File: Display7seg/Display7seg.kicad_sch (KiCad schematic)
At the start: 6 parts

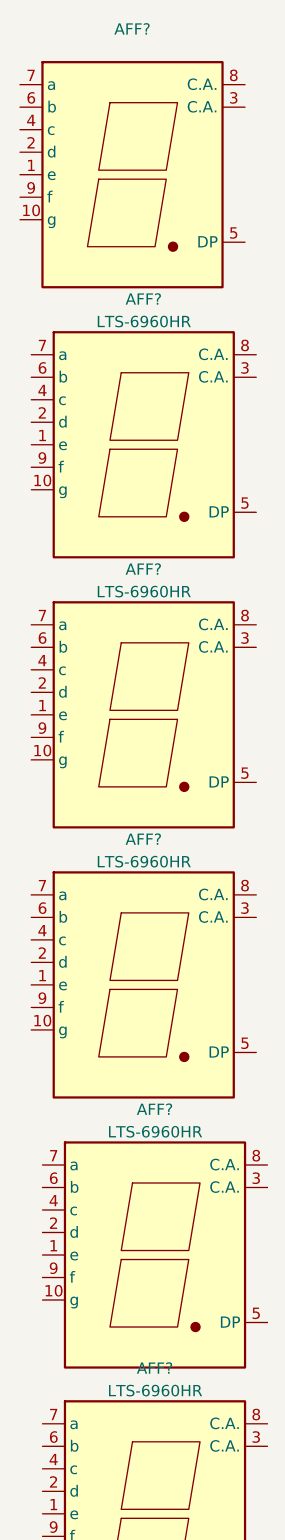
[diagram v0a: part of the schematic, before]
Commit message: Display
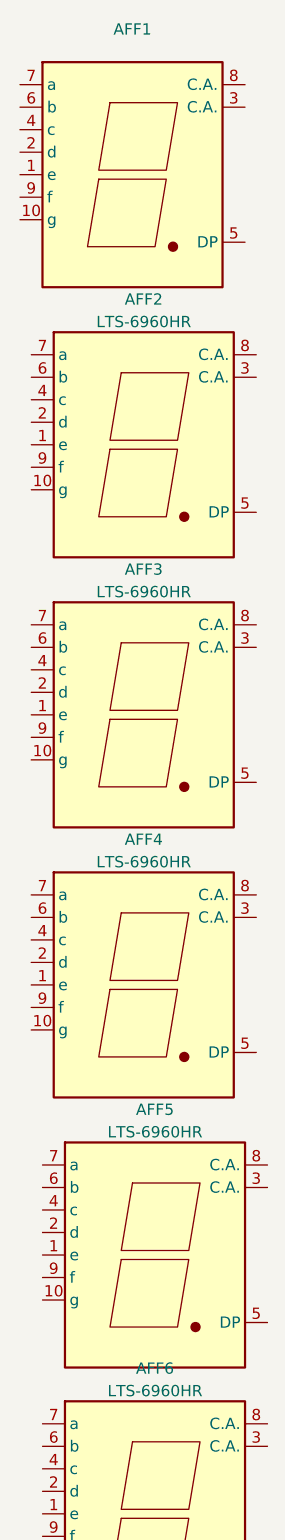
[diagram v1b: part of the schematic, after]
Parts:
- gave numbers to parts that had none: 6
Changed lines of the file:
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@@
   (symbol (lib_id "Display_Character:LTS-6960HR") (at 120.65 152.4 0) (unit 1)
     (in_bom yes) (on_board yes) (fields_autoplaced)
-    (property "Reference" "AFF?" (id 0) (at 120.65 136.0002 0))
+    (property "Reference" "AFF5" (id 0) (at 120.65 136.0002 0))
     (property "Value" "LTS-6960HR" (id 1) (at 120.65 138.5371 0))
     (property "Footprint" "Display_7Segment:7SegmentLED_LTS6760_LTS6780" (id 2) (at 120.65 167.64 0)
@@
   (symbol (lib_id "Display_Character:LTS-6960HR") (at 119.38 60.96 0) (unit 1)
     (in_bom yes) (on_board yes) (fields_autoplaced)
-    (property "Reference" "AFF?" (id 0) (at 119.38 44.5602 0))
+    (property "Reference" "AFF2" (id 0) (at 119.38 44.5602 0))
     (property "Value" "LTS-6960HR" (id 1) (at 119.38 47.0971 0))
     (property "Footprint" "Display_7Segment:7SegmentLED_LTS6760_LTS6780" (id 2) (at 119.38 76.2 0)
@@
   (symbol (lib_id "Display_Character:LTS-6960HR") (at 120.65 181.61 0) (unit 1)
     (in_bom yes) (on_board yes) (fields_autoplaced)
-    (property "Reference" "AFF?" (id 0) (at 120.65 165.2102 0))
+    (property "Reference" "AFF6" (id 0) (at 120.65 165.2102 0))
     (property "Value" "LTS-6960HR" (id 1) (at 120.65 167.7471 0))
     (property "Footprint" "Display_7Segment:7SegmentLED_LTS6760_LTS6780" (id 2) (at 120.65 196.85 0)
@@
   (symbol (lib_id "Display_Character:LTS-6960HR") (at 119.38 91.44 0) (unit 1)
     (in_bom yes) (on_board yes) (fields_autoplaced)
-    (property "Reference" "AFF?" (id 0) (at 119.38 75.0402 0))
+    (property "Reference" "AFF3" (id 0) (at 119.38 75.0402 0))
     (property "Value" "LTS-6960HR" (id 1) (at 119.38 77.5771 0))
     (property "Footprint" "Display_7Segment:7SegmentLED_LTS6760_LTS6780" (id 2) (at 119.38 106.68 0)
@@
   (symbol (lib_id "Display_Character:LTS-6960HR") (at 118.11 30.48 0) (unit 1)
     (in_bom yes) (on_board yes) (fields_autoplaced)
-    (property "Reference" "AFF?" (id 0) (at 118.11 14.0802 0))
+    (property "Reference" "AFF1" (id 0) (at 118.11 14.0802 0))
     (property "Value" "" (id 1) (at 118.11 16.6171 0))
     (property "Footprint" "" (id 2) (at 118.11 45.72 0)
@@
   (symbol (lib_id "Display_Character:LTS-6960HR") (at 119.38 121.92 0) (unit 1)
     (in_bom yes) (on_board yes) (fields_autoplaced)
-    (property "Reference" "AFF?" (id 0) (at 119.38 105.5202 0))
+    (property "Reference" "AFF4" (id 0) (at 119.38 105.5202 0))
     (property "Value" "LTS-6960HR" (id 1) (at 119.38 108.0571 0))
     (property "Footprint" "Display_7Segment:7SegmentLED_LTS6760_LTS6780" (id 2) (at 119.38 137.16 0)
@@
   )
   (symbol_instances
-    (path "/037e3cea-2b4e-4a8e-b505-8a054542ddbd"
-      (reference "AFF?") (unit 1) (value "LTS-6960HR") (footprint "Display_7Segment:7SegmentLED_LTS6760_LTS6780")
+    (path "/e82a6e2d-1a74-4e83-87b6-27ce032478fa"
+      (reference "AFF1") (unit 1) (value "LTS-6960HR") (footprint "Display_7Segment:7SegmentLED_LTS6760_LTS6780")
     )
     (path "/231a3042-ec36-4c9a-bd14-ea32ea232394"
-      (reference "AFF?") (unit 1) (value "LTS-6960HR") (footprint "Display_7Segment:7SegmentLED_LTS6760_LTS6780")
+      (reference "AFF2") (unit 1) (value "LTS-6960HR") (footprint "Display_7Segment:7SegmentLED_LTS6760_LTS6780")
+    )
+    (path "/9cad7174-bb88-4cff-8061-48eaf01fef6d"
+      (reference "AFF3") (unit 1) (value "LTS-6960HR") (footprint "Display_7Segment:7SegmentLED_LTS6760_LTS6780")
+    )
+    (path "/f1ee0cd5-9267-462c-9d04-1dd00febaf6c"
+      (reference "AFF4") (unit 1) (value "LTS-6960HR") (footprint "Display_7Segment:7SegmentLED_LTS6760_LTS6780")
+    )
+    (path "/037e3cea-2b4e-4a8e-b505-8a054542ddbd"
+      (reference "AFF5") (unit 1) (value "LTS-6960HR") (footprint "Display_7Segment:7SegmentLED_LTS6760_LTS6780")
     )
     (path "/2b76cefd-3e5b-46ea-aeb2-6a2b85d260ff"
-      (reference "AFF?") (unit 1) (value "LTS-6960HR") (footprint "Display_7Segment:7SegmentLED_LTS6760_LTS6780")
-    )
-    (path "/9cad7174-bb88-4cff-8061-48eaf01fef6d"
-      (reference "AFF?") (unit 1) (value "LTS-6960HR") (footprint "Display_7Segment:7SegmentLED_LTS6760_LTS6780")
-    )
-    (path "/e82a6e2d-1a74-4e83-87b6-27ce032478fa"
-      (reference "AFF?") (unit 1) (value "LTS-6960HR") (footprint "Display_7Segment:7SegmentLED_LTS6760_LTS6780")
-    )
-    (path "/f1ee0cd5-9267-462c-9d04-1dd00febaf6c"
-      (reference "AFF?") (unit 1) (value "LTS-6960HR") (footprint "Display_7Segment:7SegmentLED_LTS6760_LTS6780")
+      (reference "AFF6") (unit 1) (value "LTS-6960HR") (footprint "Display_7Segment:7SegmentLED_LTS6760_LTS6780")
     )
   )

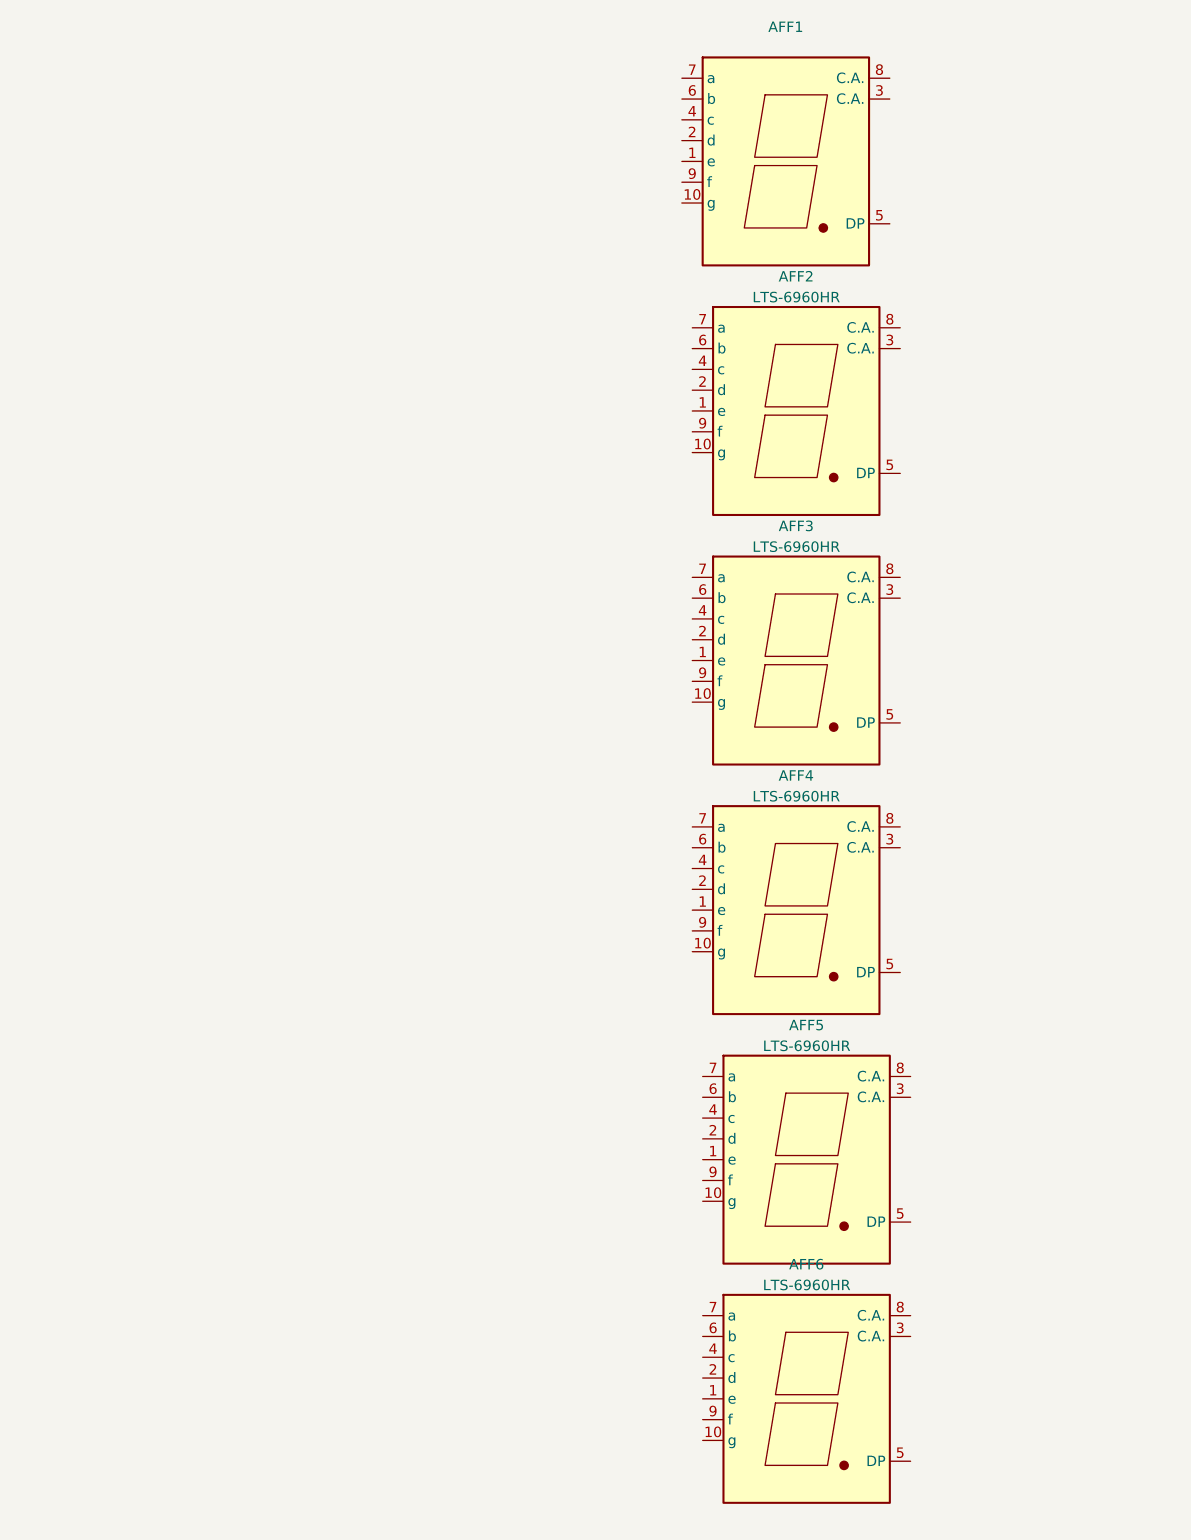
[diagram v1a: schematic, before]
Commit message: REFACTOR
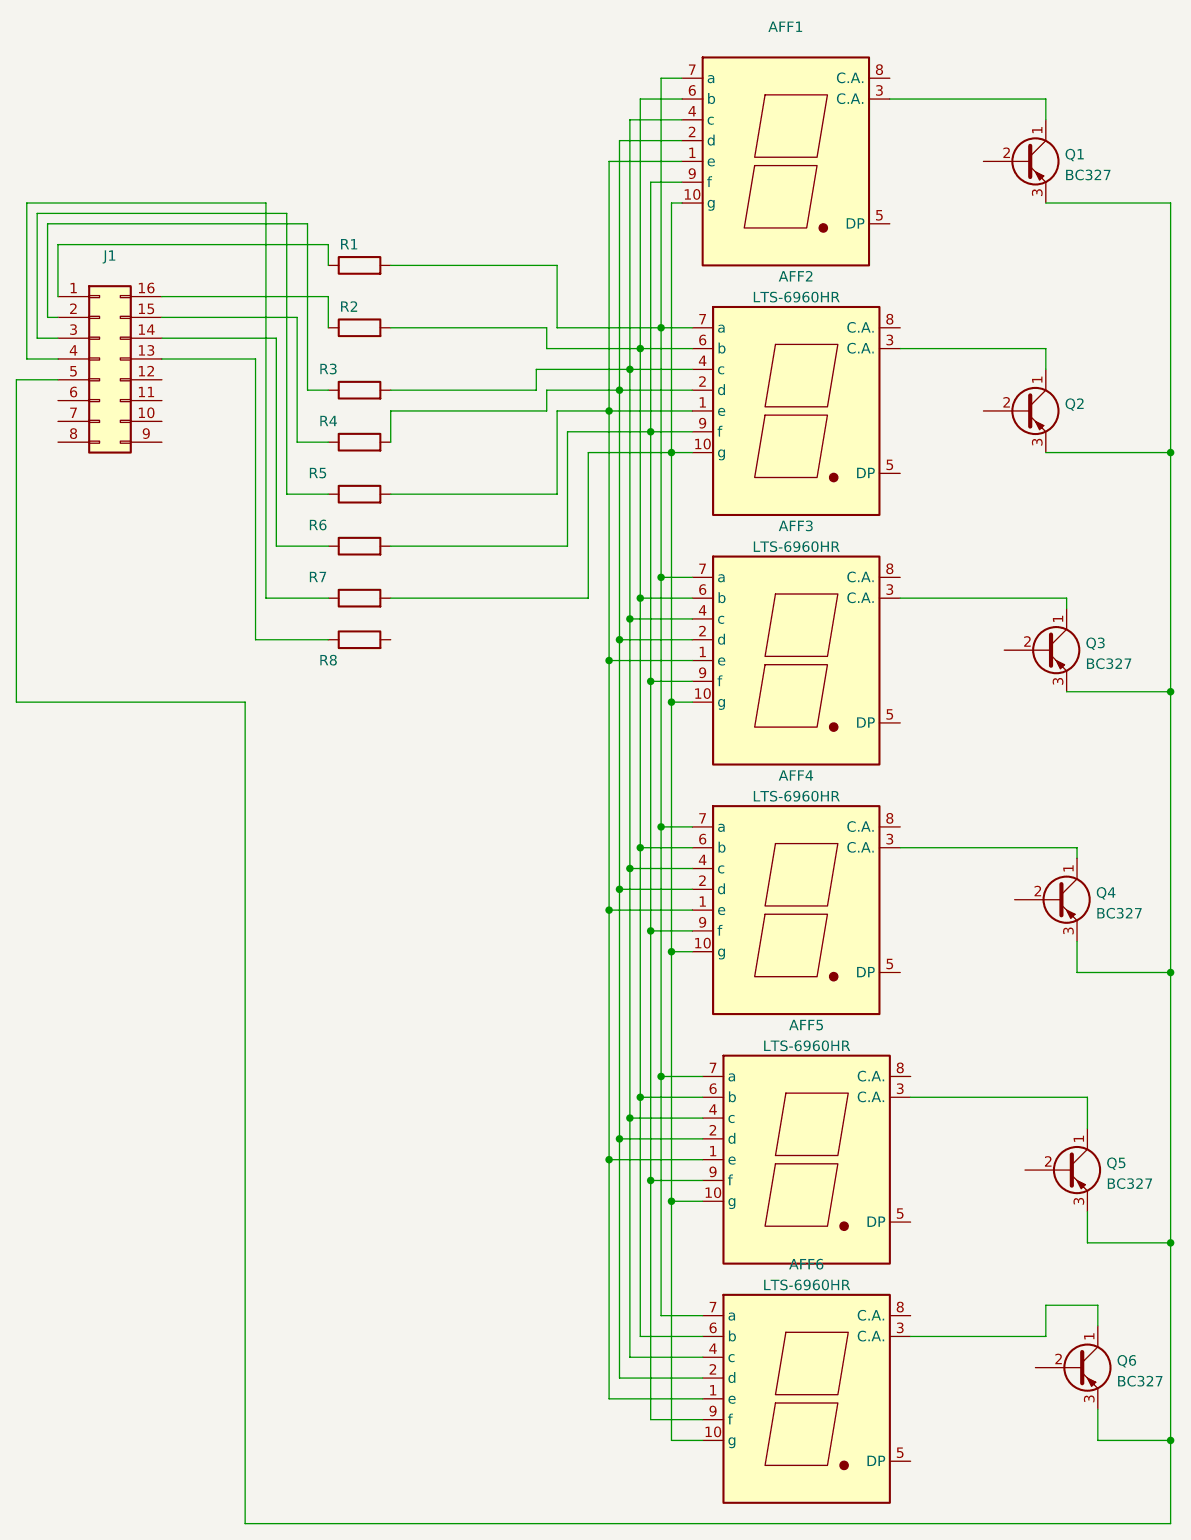
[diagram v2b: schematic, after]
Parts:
- added J1: (no value), symbol Connector_Generic:Conn_02x08_Counter_Clockwise
- added Q1, Q3, Q4, Q5, Q6: BC327, Package_TO_SOT_THT:TO-92_Inline, symbol Transistor_BJT:BC327
- added Q2: (no value), symbol Transistor_BJT:BC327
- added R1, R2, R3, R4, R5, R6, R7, R8: (no value), symbol Device:R
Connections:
- net at AFF5.1 (e): now also AFF1.1 (e), AFF2.1 (e), AFF3.1 (e), AFF4.1 (e), AFF6.1 (e), R5.2
- net at AFF5.10 (g): now also AFF1.10 (g), AFF2.10 (g), AFF3.10 (g), AFF4.10 (g), AFF6.10 (g), R7.2
- net at AFF5.2 (d): now also AFF1.2 (d), AFF2.2 (d), AFF3.2 (d), AFF4.2 (d), AFF6.2 (d), R4.2
- net at AFF5.3 (C.A.): now also Q5.1 (C)
- net at AFF5.4 (c): now also AFF1.4 (c), AFF2.4 (c), AFF3.4 (c), AFF4.4 (c), AFF6.4 (c), R3.2
- net at AFF5.6 (b): now also AFF1.6 (b), AFF2.6 (b), AFF3.6 (b), AFF4.6 (b), AFF6.6 (b), R2.2
- net at AFF5.7 (a): now also AFF1.7 (a), AFF2.7 (a), AFF3.7 (a), AFF4.7 (a), AFF6.7 (a), R1.2
- net at AFF5.9 (f): now also AFF1.9 (f), AFF2.9 (f), AFF3.9 (f), AFF4.9 (f), AFF6.9 (f), R6.2
- net at AFF2.3 (C.A.): now also Q2.1 (C)
- net at AFF6.3 (C.A.): now also Q6.1 (C)
- net at AFF3.3 (C.A.): now also Q3.1 (C)
- net at AFF1.3 (C.A.): now also Q1.1 (C)
- net at AFF4.3 (C.A.): now also Q4.1 (C)
- new net: J1.3 (Pin_3), R5.1
- new net: J1.2 (Pin_2), R3.1
- new net: J1.5 (Pin_5), Q1.3 (E), Q2.3 (E), Q3.3 (E), Q4.3 (E), Q5.3 (E), Q6.3 (E)
- new net: J1.4 (Pin_4), R7.1
- new net: J1.16 (Pin_16), R2.1
- new net: J1.1 (Pin_1), R1.1
- new net: J1.13 (Pin_13), R8.1
- new net: J1.14 (Pin_14), R6.1
- new net: J1.15 (Pin_15), R4.1
